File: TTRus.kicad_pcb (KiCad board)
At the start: 2 copper layers, 79.5 x 80.5 mm, 1 part

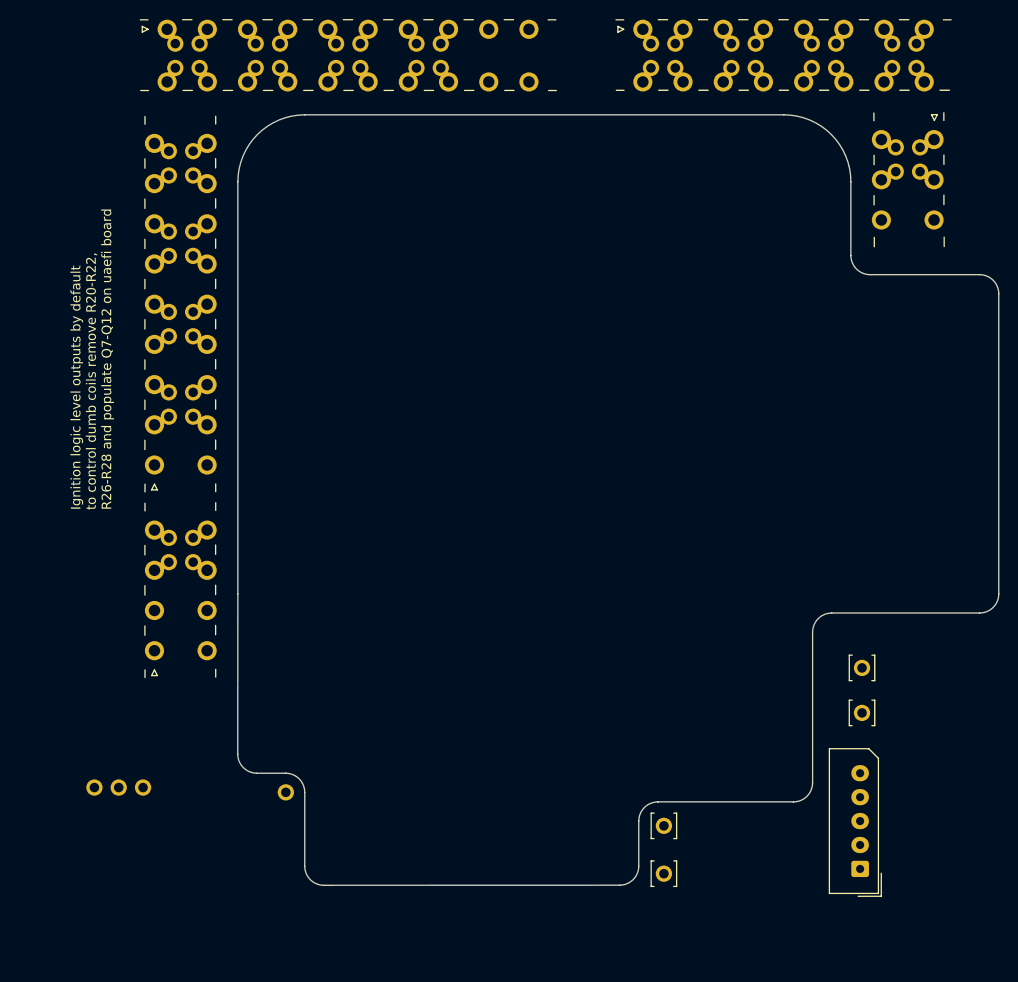
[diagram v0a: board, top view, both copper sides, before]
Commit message: Add files via upload
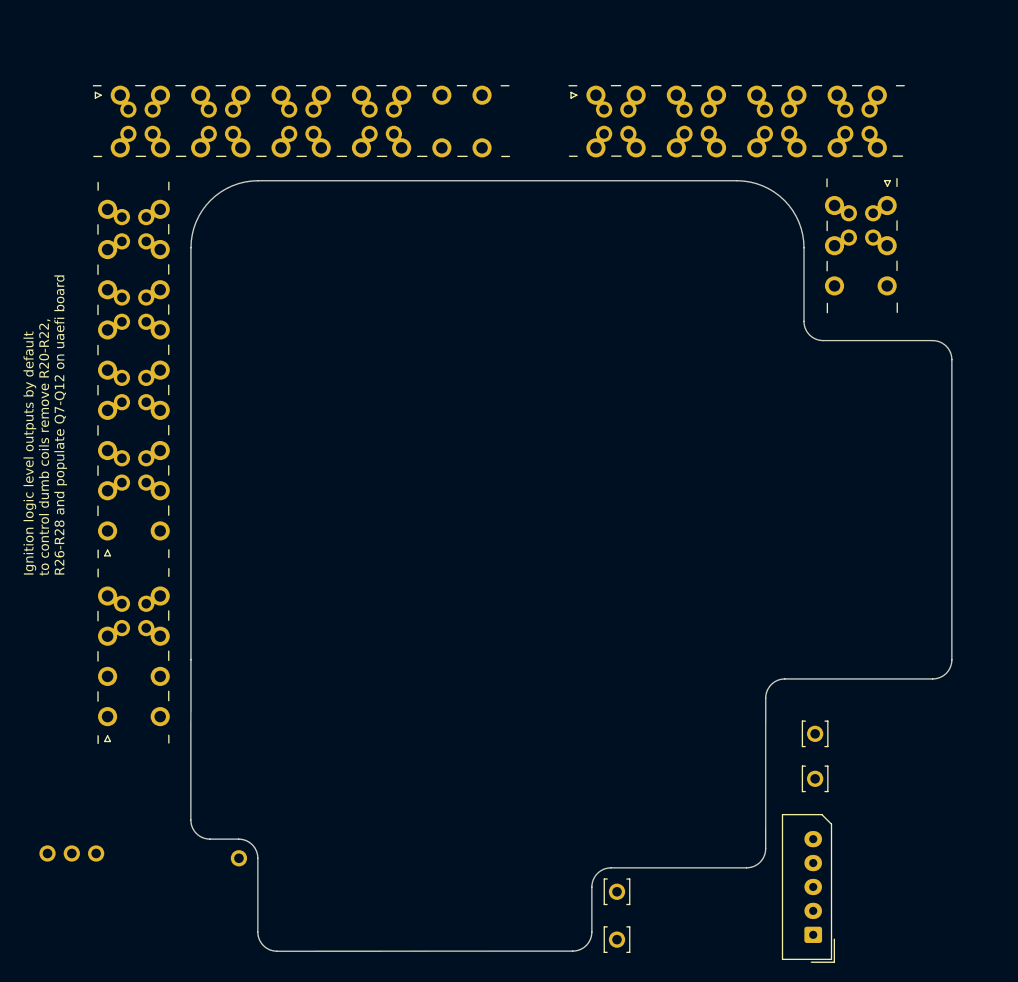
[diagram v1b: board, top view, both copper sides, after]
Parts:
- removed REF**: UAEFI_BRD, Hellen:uaefi
- added M1: Module:uaefi/0.2, Hellen:uaefi, F.Cu at (89.1, 143.9)
